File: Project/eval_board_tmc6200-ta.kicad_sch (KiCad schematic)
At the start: 0 parts

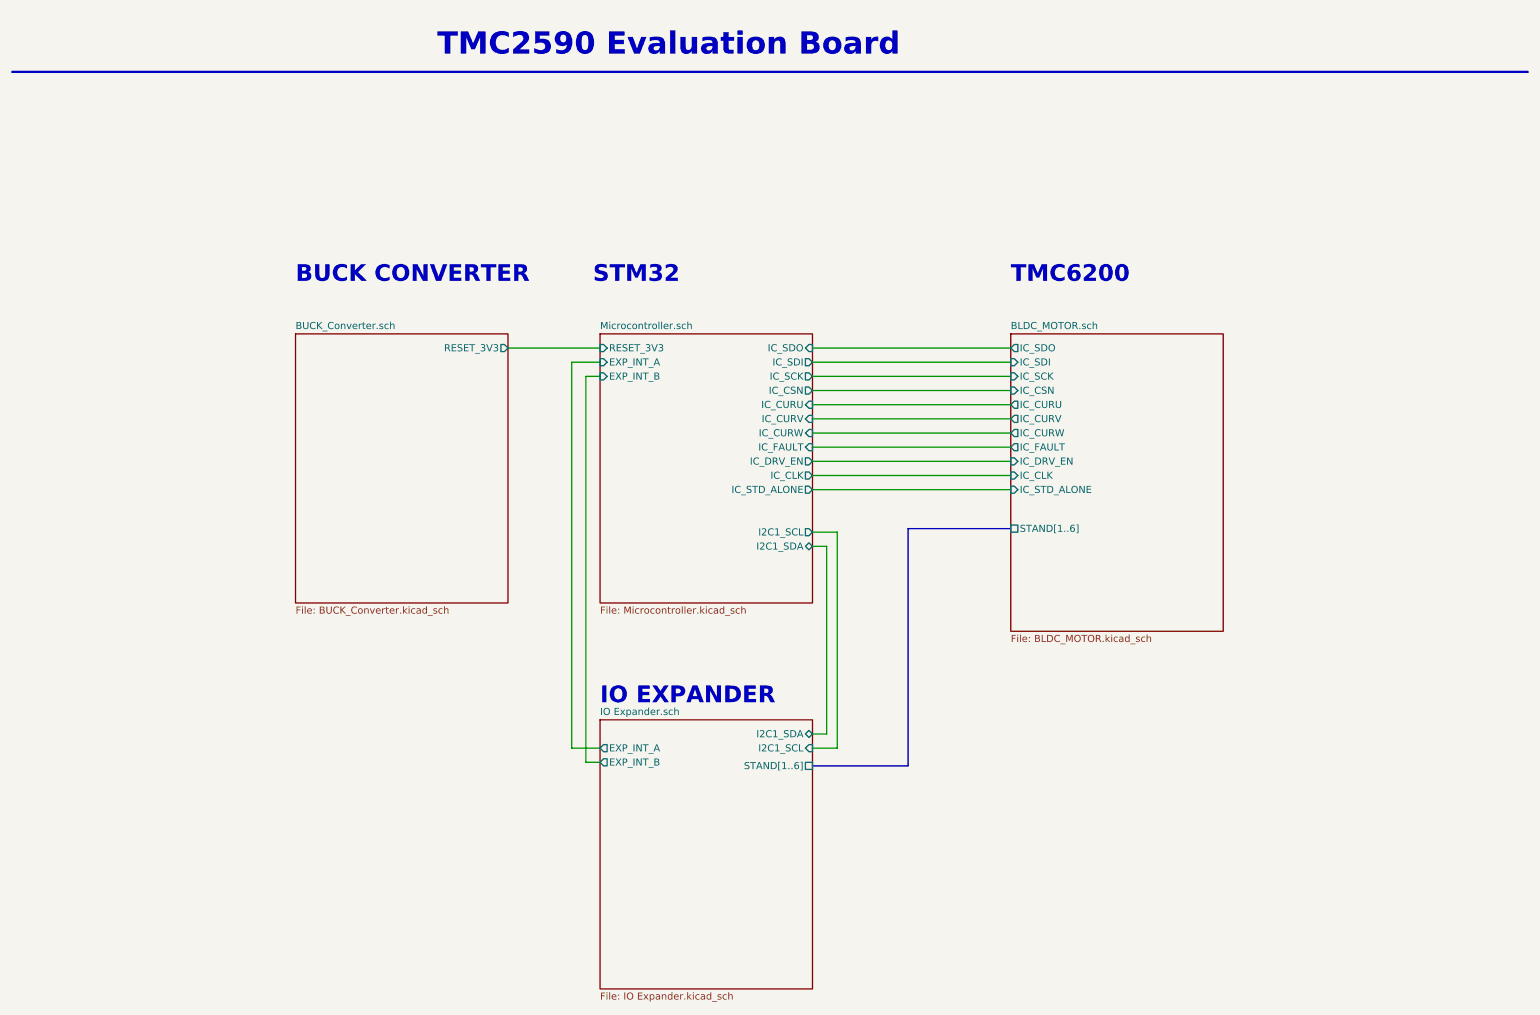
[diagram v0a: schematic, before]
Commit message: Cleanup ED A1 version
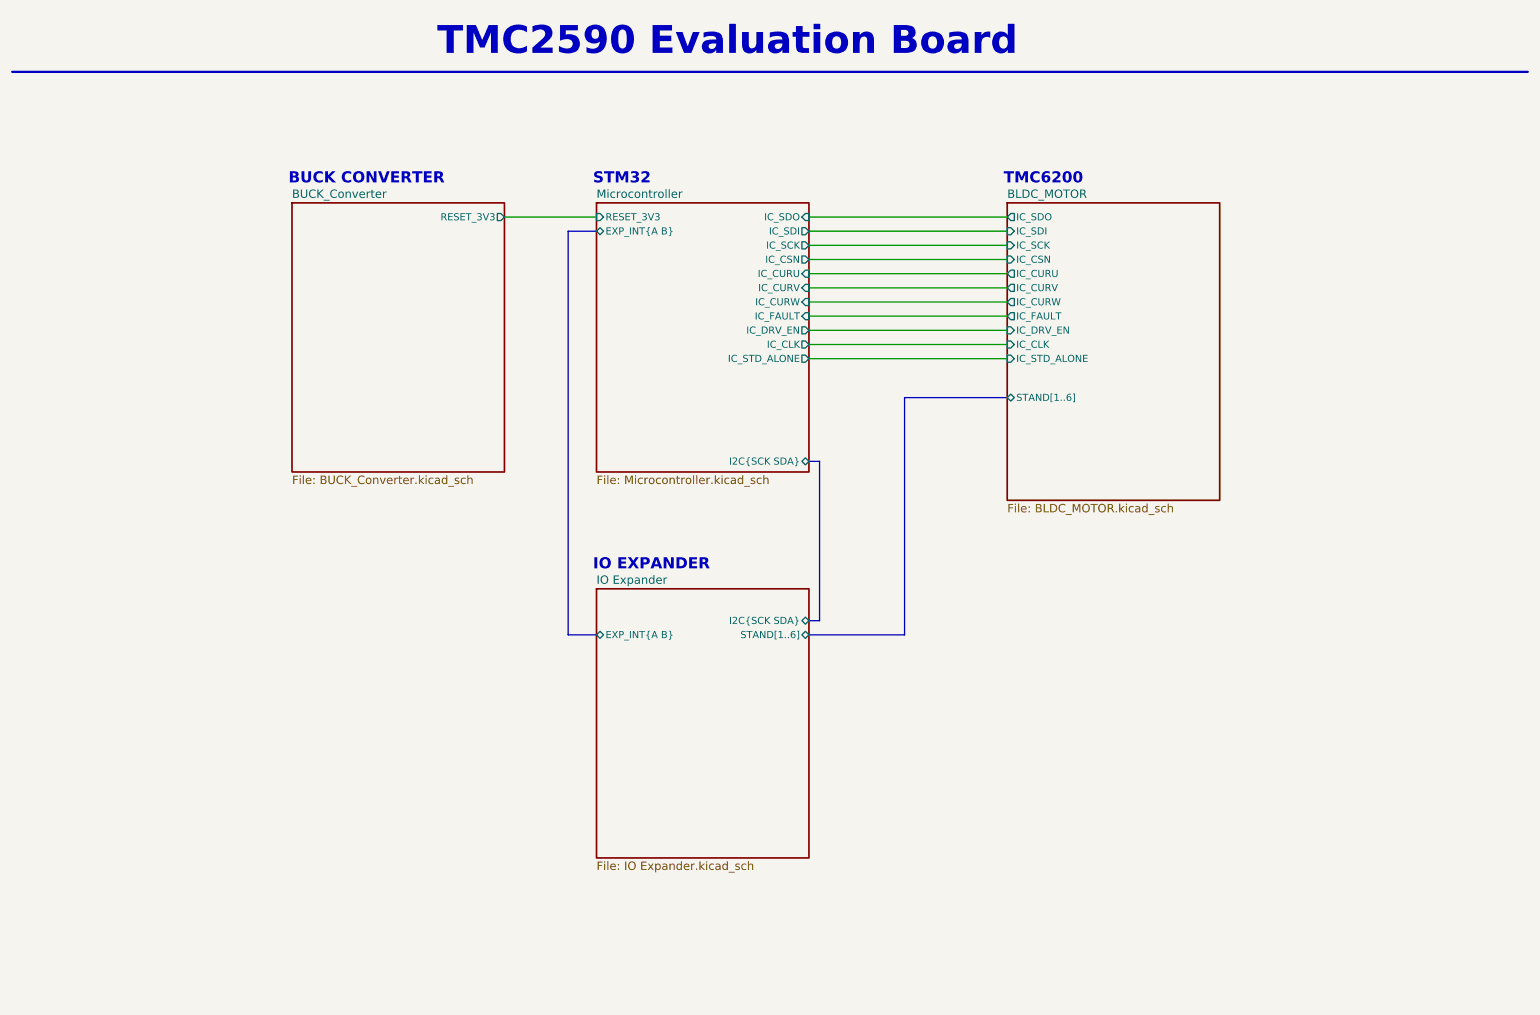
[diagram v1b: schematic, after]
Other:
- sheet BLDC_MOTOR.sch renamed BLDC_MOTOR
- sheet BUCK_Converter.sch renamed BUCK_Converter
- sheet IO Expander.sch renamed IO Expander
- sheet Microcontroller.sch renamed Microcontroller
- sheet IO Expander ports: added EXP_INT{A B}, I2C{SCK SDA}; removed EXP_INT_A, EXP_INT_B, I2C1_SCL, I2C1_SDA
- sheet Microcontroller ports: added EXP_INT{A B}, I2C{SCK SDA}; removed EXP_INT_A, EXP_INT_B, I2C1_SCL, I2C1_SDA
